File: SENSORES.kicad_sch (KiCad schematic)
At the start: 7 parts, among them U4 BMI088

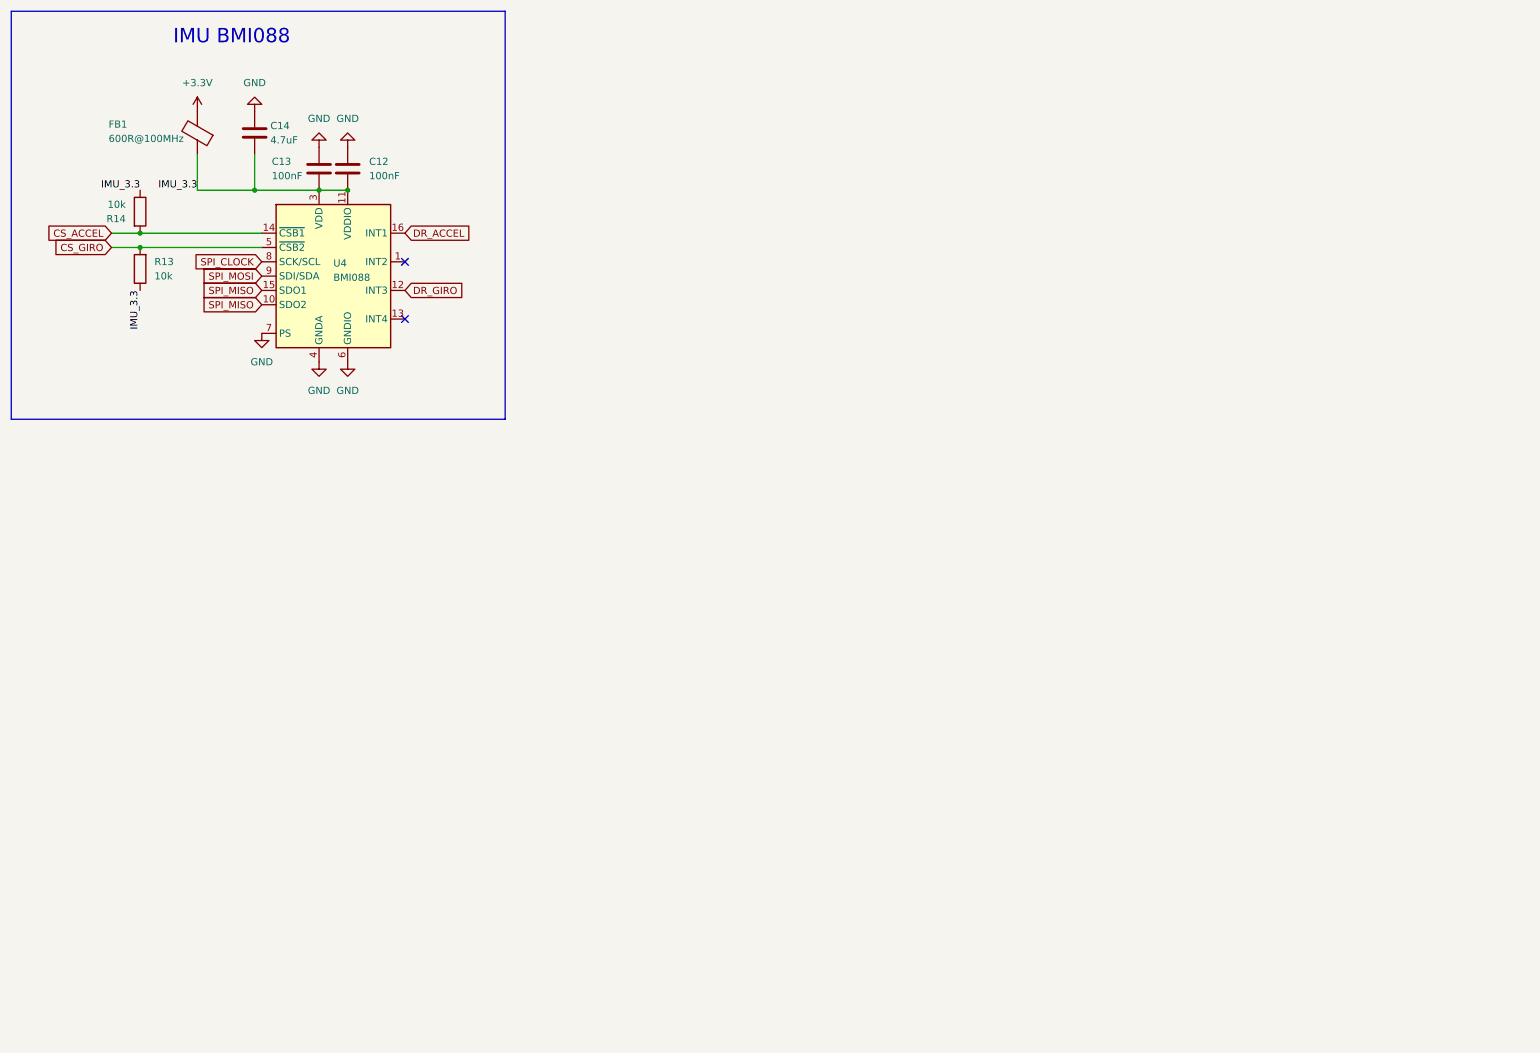
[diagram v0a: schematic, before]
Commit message: Esquematico preparado para revision
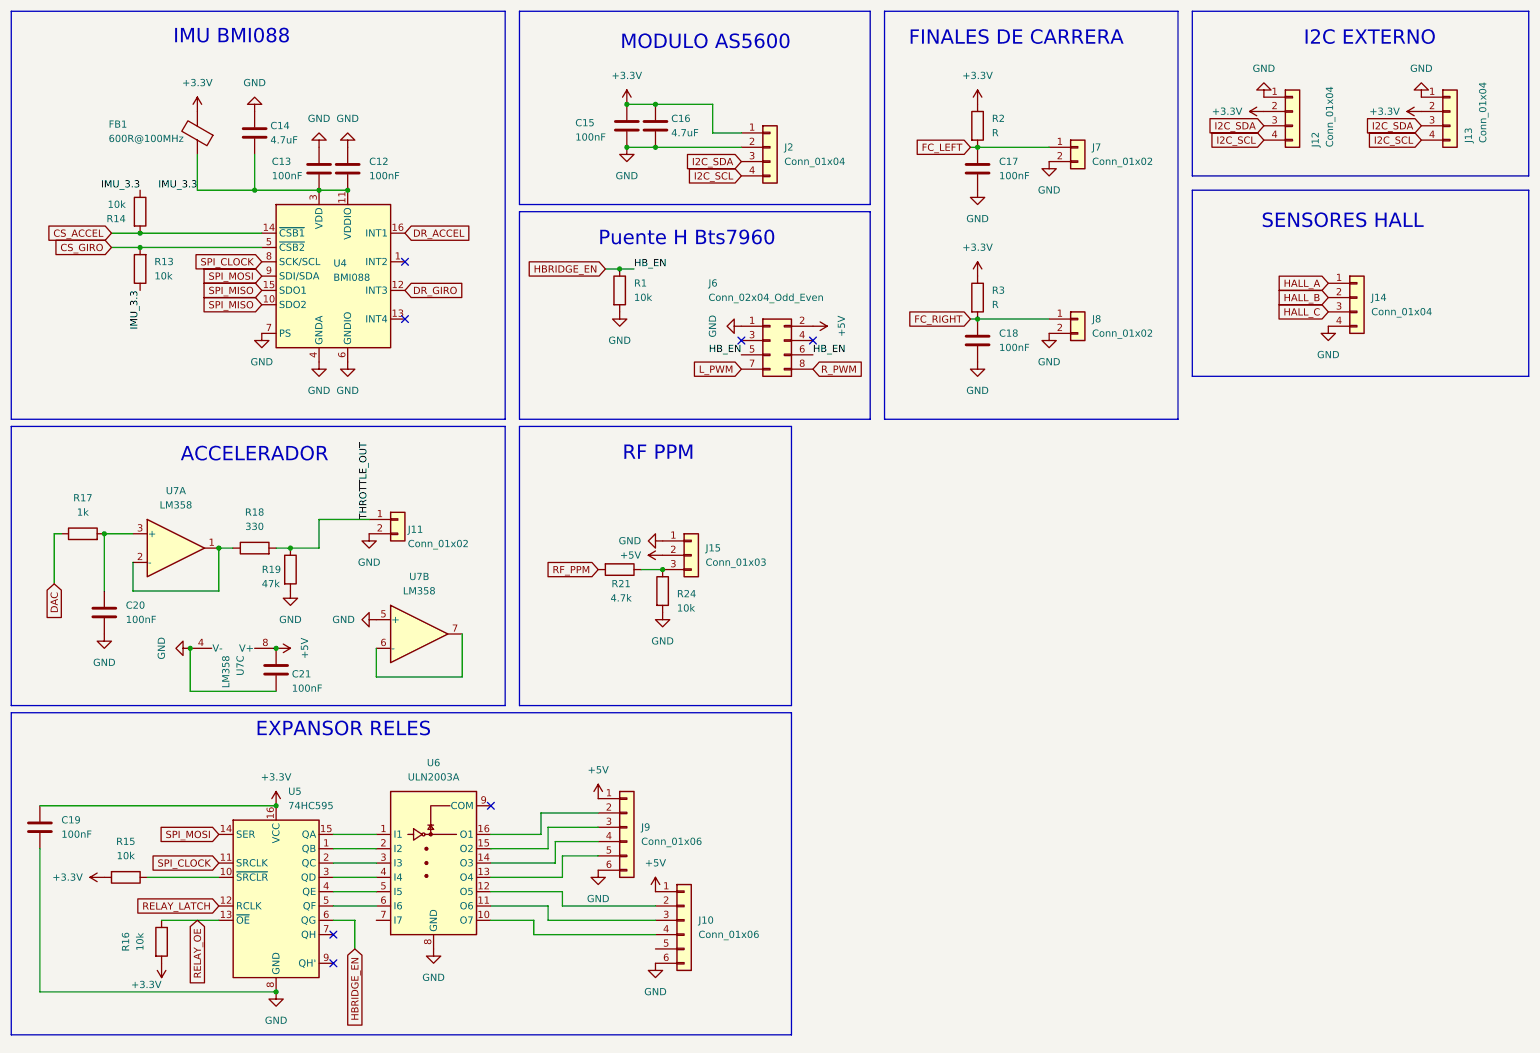
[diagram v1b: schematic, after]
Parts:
- added C15: 100nF, Capacitor_SMD:C_0603_1608Metric, symbol Device:C
- added C16: 4.7uF, Capacitor_SMD:C_0805_2012Metric, symbol Device:C
- added C17, C18, C19, C20, C21: 100nF, symbol Device:C
- added J10, J9: Conn_01x06, symbol Connector_Generic:Conn_01x06
- added J11, J7, J8: Conn_01x02, symbol Connector_Generic:Conn_01x02
- added J12, J13, J14, J2: Conn_01x04, symbol Connector_Generic:Conn_01x04
- added J15: Conn_01x03, symbol Connector_Generic:Conn_01x03
- added J6: Conn_02x04_Odd_Even, symbol Connector_Generic:Conn_02x04_Odd_Even
- added R1, R15, R16, R24: 10k, symbol Device:R
- added R17: 1k, symbol Device:R
- added R18: 330, symbol Device:R
- added R19: 47k, symbol Device:R
- added R2, R3: R, symbol Device:R
- added R21: 4.7k, symbol Device:R
- added U5: 74HC595, symbol 74xx:74HC595
- added U6: ULN2003A, symbol Transistor_Array:ULN2003A
- added U7: LM358, symbol Amplifier_Operational:LM358
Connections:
- net +3.3V: now also C15.2, C16.1, C19.1, J12.2 (Pin_2), J13.2 (Pin_2), J2.1 (Pin_1), R15.2, R16.2, R2.1, R3.1, U5.16 (VCC)
- net GND: now also C15.1, C16.2, C17.2, C18.2, C19.2, C20.2, C21.2, J10.6 (Pin_6), J11.2 (Pin_2), J12.1 (Pin_1), J13.1 (Pin_1), J14.4 (Pin_4), J15.1 (Pin_1), J2.2 (Pin_2), J6.1 (Pin_1), J7.2 (Pin_2), J8.2 (Pin_2), J9.6 (Pin_6), R1.2, R19.2, R24.2, U5.8 (GND), U6.8 (GND), U7.4 (V-), U7.5 (+)
- net SPI_CLOCK: now also U5.11 (SRCLK)
- net SPI_MOSI: now also U5.14 (SER)
- new net: C20.1, R17.2, U7.3 (+)
- new net: J9.2 (Pin_2), U6.16 (O1)
- new net: J9.3 (Pin_3), U6.15 (O2)
- new net: J9.4 (Pin_4), U6.14 (O3)
- new net: J9.5 (Pin_5), U6.13 (O4)
- new net: J15.3 (Pin_3), R21.1, R24.1
- new net: U5.15 (QA), U6.1 (I1)
- new net: J10.4 (Pin_4), U6.10 (O7)
- new net: J10.3 (Pin_3), U6.11 (O6)
- new net: J10.2 (Pin_2), U6.12 (O5)
- new net: U5.1 (QB), U6.2 (I2)
- new net: U5.2 (QC), U6.3 (I3)
- new net: U5.3 (QD), U6.4 (I4)
- new net: U5.4 (QE), U6.5 (I5)
- new net: U5.5 (QF), U6.6 (I6)
- new net: R15.1, U5.10 (~{SRCLR})
- new net: R18.1, U7.1, U7.2 (-)
- new net: U7.6 (-), U7.7
- new net +5V: C21.1, J10.1 (Pin_1), J15.2 (Pin_2), J6.2 (Pin_2), J9.1 (Pin_1), U7.8 (V+)
- new net DAC: R17.1
- new net FC_LEFT: C17.1, J7.1 (Pin_1), R2.2
- new net FC_RIGHT: C18.1, J8.1 (Pin_1), R3.2
- new net HALL_A: J14.1 (Pin_1)
- new net HALL_B: J14.2 (Pin_2)
- new net HALL_C: J14.3 (Pin_3)
- new net HBRIDGE_EN: J6.5 (Pin_5), J6.6 (Pin_6), R1.1, U5.6 (QG)
- new net I2C_SCL: J12.4 (Pin_4), J13.4 (Pin_4), J2.4 (Pin_4)
- new net I2C_SDA: J12.3 (Pin_3), J13.3 (Pin_3), J2.3 (Pin_3)
- new net L_PWM: J6.7 (Pin_7)
- new net RELAY_LATCH: U5.12 (RCLK)
- new net RELAY_OE: R16.1, U5.13 (~{OE})
- new net RF_PPM: R21.2
- new net R_PWM: J6.8 (Pin_8)
- new net THROTTLE_OUT: J11.1 (Pin_1), R18.2, R19.1
- no-connect marks 2 -> 7
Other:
- note added: "ACCELERADOR"
- note added: "EXPANSOR RELES"
- note added: "FINALES DE CARRERA"
- note added: "I2C EXTERNO"
- note added: "MODULO AS5600"
- note added: "Puente H Bts7960"
- note added: "RF PPM"
- note added: "SENSORES HALL"
